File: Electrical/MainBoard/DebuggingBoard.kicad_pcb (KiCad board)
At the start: 6 copper layers, 120 x 80 mm, 179 parts, among them J1 Barrel_Jack_Switch, Q1 AO3401A, SW1 SW_SPDT, U1 CH224K, U10 FFC2B28-24-G, U11 SM08B-PASS-TBT(LF)(SN), U12 SM05B-PASS-TBT(LF)(SN), U13 SM02B-PASS-TBT(LF)(SN), U14 SM06B-PASS-TBT(LF)(SN), U15 SM05B-PASS-TBT(LF)(SN), U16 SM05B-PASS-TBT(LF)(SN), U17 SM05B-PASS-TBT(LF)(SN), U2 STM32H723VGTx, U3 APS6404L-3SQR-ZR, U4 USB3300-EZK, U5 TPS65131RGE, U6 TPS2121RUXR, U7 TPS7A9401DSCR, U8 LM61460AASQRJRRQ1, U9 S5B-ZR-SM4A-TF(LF)(SN), Y1 X322525MOB4SI, Y2 X322524MOB4SI

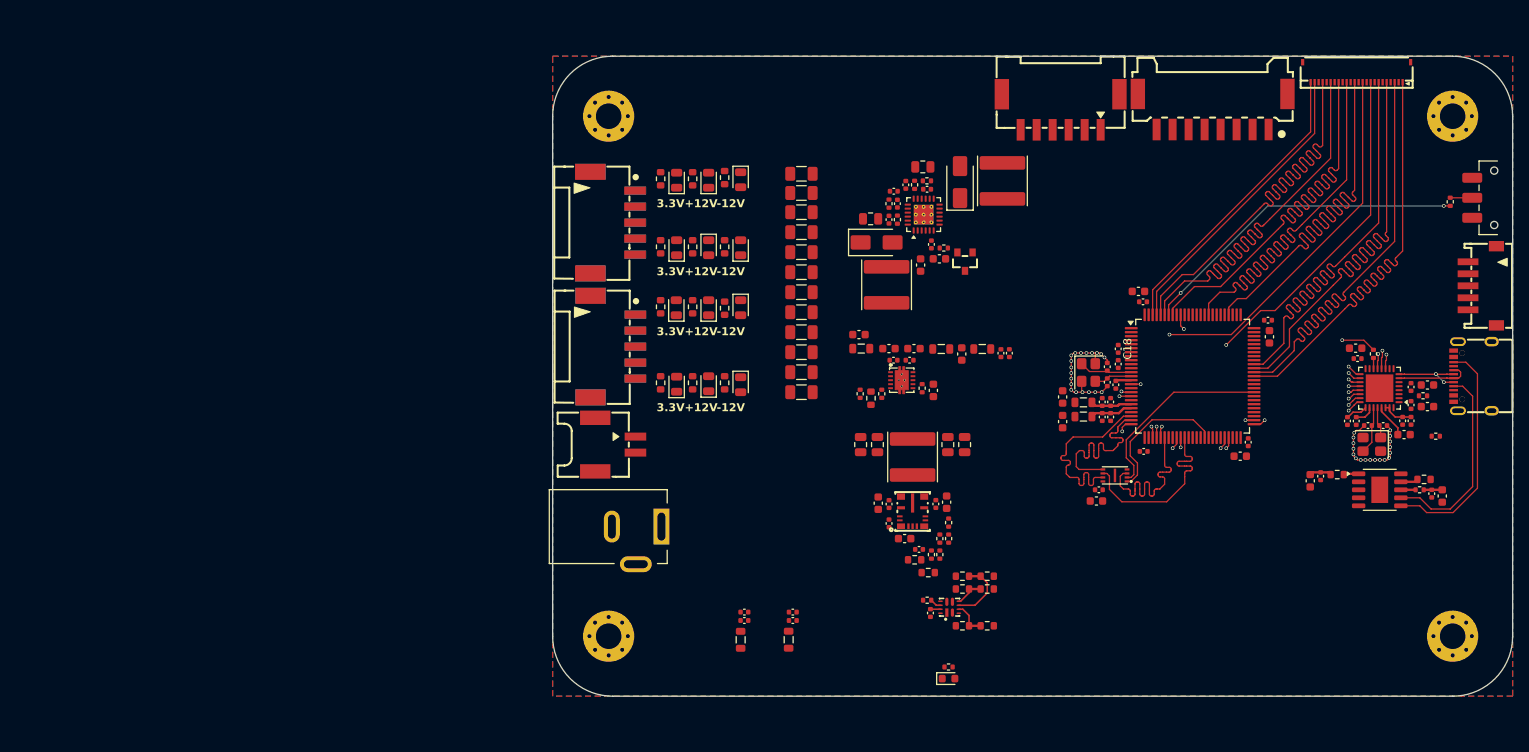
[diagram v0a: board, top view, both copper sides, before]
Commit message: new layout
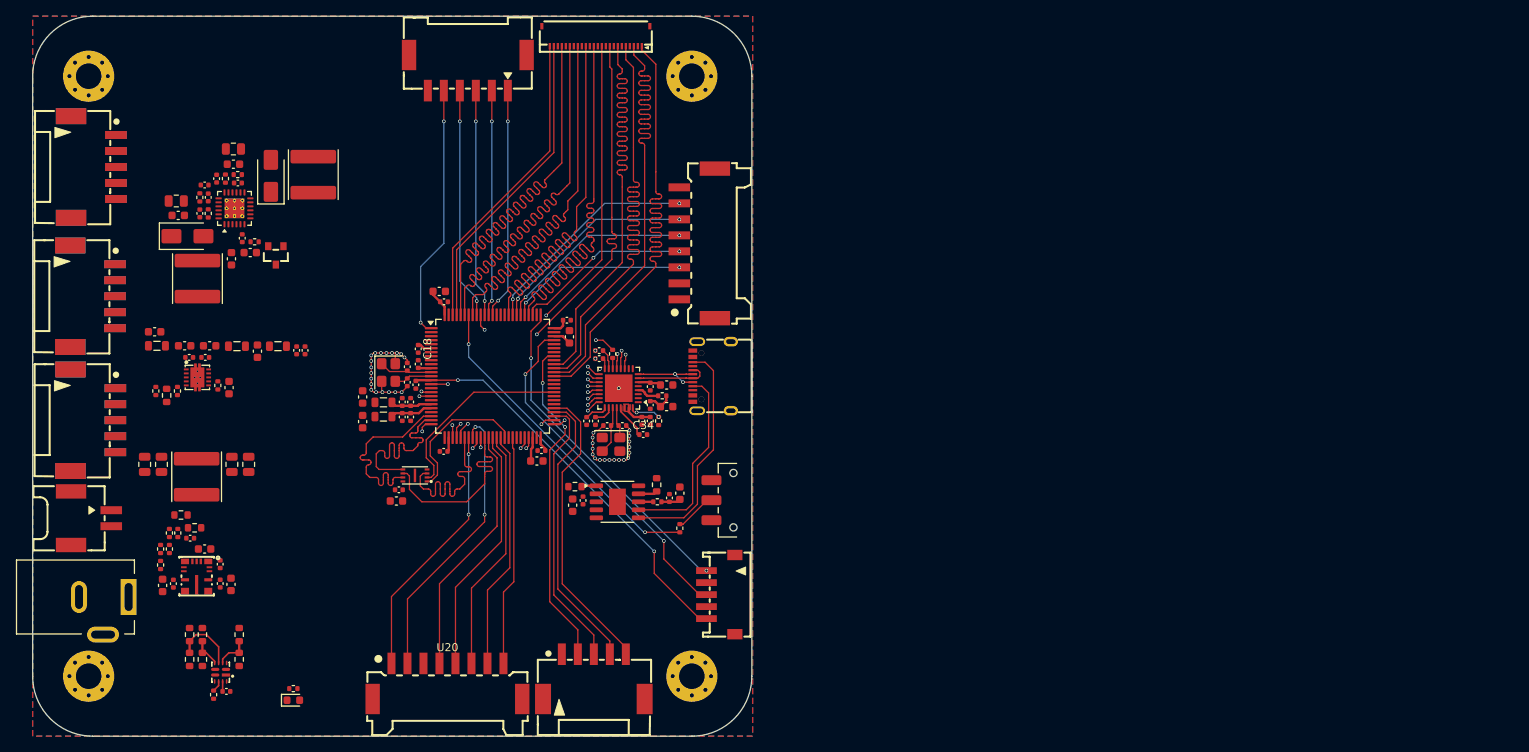
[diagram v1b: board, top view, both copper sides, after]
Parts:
- removed C57, C58: 10nF, Capacitor_SMD:C_0402_1005Metric
- removed D10, D11, D12, D13, D14, D15, D4, D5, D6, D7, D8, D9: LED, LED_SMD:LED_0805_2012Metric
- removed F1, F10, F11, F12, F2, F3, F4, F5, F6, F7, F8, F9: 500MA/24V, Fuse:Fuse_1206_3216Metric
- removed FB5, FB7: 600R@100MHz, Inductor_SMD:L_0805_2012Metric
- removed R32, R37, R40, R43: 330R, Resistor_SMD:R_0603_1608Metric
- removed R33, R34, R35, R36, R38, R39, R41, R42: 2.2K, Resistor_SMD:R_0603_1608Metric
- added U18: SM05B-PASS-TBT(LF)(SN), JLC_PARTS:CONN-SMD_5P-P2.00_SM05B-PASS-TBT-LF-SN, F.Cu at (77.6, 63.8)
- added U19: SM05B-PASS-TBT(LF)(SN), JLC_PARTS:CONN-SMD_5P-P2.00_SM05B-PASS-TBT-LF-SN, B.Cu at (77.6, 63.9)
- added U20: SM08B-PASS-TBT(LF)(SN), JLC_PARTS:CONN-SMD_SM08B-PASS-TBT-LF-SN, F.Cu at (121.9, 128.1)
- added U21: SM05B-PASS-TBT(LF)(SN), JLC_PARTS:CONN-SMD_5P-P2.00_SM05B-PASS-TBT-LF-SN, F.Cu at (140.1, 127.6)
- C34, C35: footprint Capacitor_SMD:C_0603_1608Metric -> Capacitor_SMD:C_0402_1005Metric
- C54, C55: value 100nF -> 1uF; footprint Capacitor_SMD:C_0402_1005Metric -> Capacitor_SMD:C_0603_1608Metric
- moved R2 104.6 mm to (150.9, 109.0)
- moved U9 102.7 mm to (156.0, 117.3)
- moved SW1 102.3 mm to (157.6, 105.5)
- moved R7 100.0 mm to (89.6, 122.3), turned to -90 degrees
- moved R24 98.6 mm to (86.0, 113.6), turned to 90 degrees
- moved C70 98.6 mm to (86.2, 116.2), turned to 90 degrees
- moved R25 98.5 mm to (86.0, 111.6), turned to 90 degrees
- moved R10 98.3 mm to (91.2, 122.3), turned to 90 degrees
- moved R8 97.2 mm to (89.6, 125.4), turned to -90 degrees
- moved R4 97.2 mm to (148.2, 95.6), turned to -90 degrees
- moved R22 96.3 mm to (87.1, 109.6), turned to 90 degrees
- moved R23 96.3 mm to (87.1, 111.6), turned to 90 degrees
- moved R1 95.9 mm to (148.0, 103.6), turned to -90 degrees
- moved C63 95.8 mm to (87.6, 115.9), turned to 90 degrees
- moved R9 95.4 mm to (91.2, 125.4), turned to 90 degrees
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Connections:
- C47 pad 2: Net-(D3-A) -> /OP_AMP-
- C50 pad 1: Net-(D2-K) -> /OP_AMP+
- C52 pad 1: Net-(D2-K) -> /OP_AMP+
- C53 pad 1: Net-(D3-A) -> /OP_AMP-
- D2 pad 1: Net-(D2-K) -> /OP_AMP+
- D3 pad 2: Net-(D3-A) -> /OP_AMP-
- R16 pad 1: Net-(D2-K) -> /OP_AMP+
- R19 pad 1: Net-(D3-A) -> /OP_AMP-
- U1 pad 10: /USB_C_PG -> unconnected-(U1-PG-Pad10)
- U11 pad 5: /DISP_NSS -> /DISP_CS
- U12 pad 1: Net-(F10-Pad2) -> +3.3V
- U12 pad 4: Net-(F11-Pad2) -> /OP_AMP+
- U12 pad 5: Net-(F12-Pad2) -> /OP_AMP-
- U15 pad 1: Net-(F1-Pad2) -> +3.3V
- U15 pad 4: Net-(F2-Pad2) -> /OP_AMP+
- U15 pad 5: Net-(F3-Pad2) -> /OP_AMP-
- U16 pad 1: Net-(F4-Pad2) -> +3.3V
- U16 pad 4: Net-(F5-Pad2) -> /OP_AMP+
- U16 pad 5: Net-(F6-Pad2) -> /OP_AMP-
- U17 pad 1: Net-(F7-Pad2) -> +3.3V
- U17 pad 4: Net-(F8-Pad2) -> /OP_AMP+
- U17 pad 5: Net-(F9-Pad2) -> /OP_AMP-
- U2 pad 1: unconnected-(U2-PE2-Pad1) -> /FGEN_SOFF
- U2 pad 32: unconnected-(U2-PC4-Pad32) -> /ADC1_INP4
- U2 pad 33: unconnected-(U2-PC5-Pad33) -> /ADC2_INP8
- U2 pad 37: unconnected-(U2-PE7-Pad37) -> /R_SRC_1K
- U2 pad 38: unconnected-(U2-PE8-Pad38) -> /R_SRC_100K
- U2 pad 39: unconnected-(U2-PE9-Pad39) -> /V_RANGE_LOW
- U2 pad 40: unconnected-(U2-PE10-Pad40) -> /V_RANGE_HIGH
- U2 pad 43: unconnected-(U2-PE13-Pad43) -> /BUZZER_CTRL
- U2 pad 53: unconnected-(U2-PB14-Pad53) -> /SPI2_MISO
- U2 pad 54: unconnected-(U2-PB15-Pad54) -> /SPI2_MOSI
- U2 pad 55: unconnected-(U2-PD8-Pad55) -> /SPI2_CS
- U2 pad 68: unconnected-(U2-PA9-Pad68) -> /SPI2_CK
- U2 pad 78: unconnected-(U2-PC10-Pad78) -> /DISP_SCK
- U2 pad 80: unconnected-(U2-PC12-Pad80) -> /DISP_MOSI
- U2 pad 81: unconnected-(U2-PD0-Pad81) -> /DISP_CS
- U2 pad 82: unconnected-(U2-PD1-Pad82) -> /DISP_DC
- U2 pad 83: unconnected-(U2-PD2-Pad83) -> /DISP_RST
- U2 pad 88: unconnected-(U2-PD7-Pad88) -> /FGEN_MOSI
- U2 pad 89: unconnected-(U2-PB3(JTDO-Pad89) -> /FGEN_SCLK
- U2 pad 90: unconnected-(U2-PB4(NJTRST)-Pad90) -> /FGEN_SAMP
- U2 pad 92: unconnected-(U2-PB6-Pad92) -> /FGEN_SGAIN
- U5 pad 15: Net-(D3-A) -> /OP_AMP-
- U5 pad 23: Net-(D2-K) -> /OP_AMP+
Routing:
- net /nRST: track 1.96 -> 50.3 mm, vias 0 -> 2
- net /SWDIO: track 0.00 -> 43.9 mm, vias 0 -> 2
- net /SWCLK: track 0.00 -> 41.9 mm, vias 0 -> 2
- net /SPI2_CK: track 0.00 -> 41.7 mm, vias 0 -> 2
- net /SPI2_CS: track 0.00 -> 37.3 mm
- net /SPI2_MOSI: track 0.00 -> 35.9 mm
- net /ADC2_INP8: track 0.00 -> 35.8 mm, vias 0 -> 2
- net /SPI2_MISO: track 0.00 -> 34.3 mm
- net /ADC1_INP4: track 0.00 -> 32.2 mm, vias 0 -> 2
- net /FGEN_SOFF: track 0.00 -> 31.8 mm, vias 0 -> 2
- net /R_SRC_1K: track 0.00 -> 31.6 mm
- net /R_SRC_100K: track 0.00 -> 31.1 mm
- net /ULPI_D7: track 49.3 -> 18.7 mm
- net /V_RANGE_LOW: track 0.00 -> 30.5 mm
- net /V_RANGE_HIGH: track 0.00 -> 29.9 mm
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- added copper zone on F.Cu, net +3.3V
- removed copper zone on In2.Cu, net GND
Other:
- board size 120 x 80 mm -> 89.9 x 90 mm
- board text removed: "+12V"
- board text removed: "-12V"
- board text removed: "3.3V"
